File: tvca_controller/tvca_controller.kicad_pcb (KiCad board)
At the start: 2 copper layers, 84.3 x 59.2 mm, 57 parts, among them J1 Programming Header, J2 PT 1,5/ 4-5,0-H, J3 4DB-P108-02, J4 PT 1,5/ 4-5,0-H, J5 4DB-P108-02, J6 PT 1,5/ 4-5,0-H, J7 4DB-P108-02, J9 4DB-P108-02, U1 PIC18F26K83, U2 MCP2562, U3 INA180, U8 VNH7070AS, U9 VNH7070AS, Y1 Crystal 12 MHz

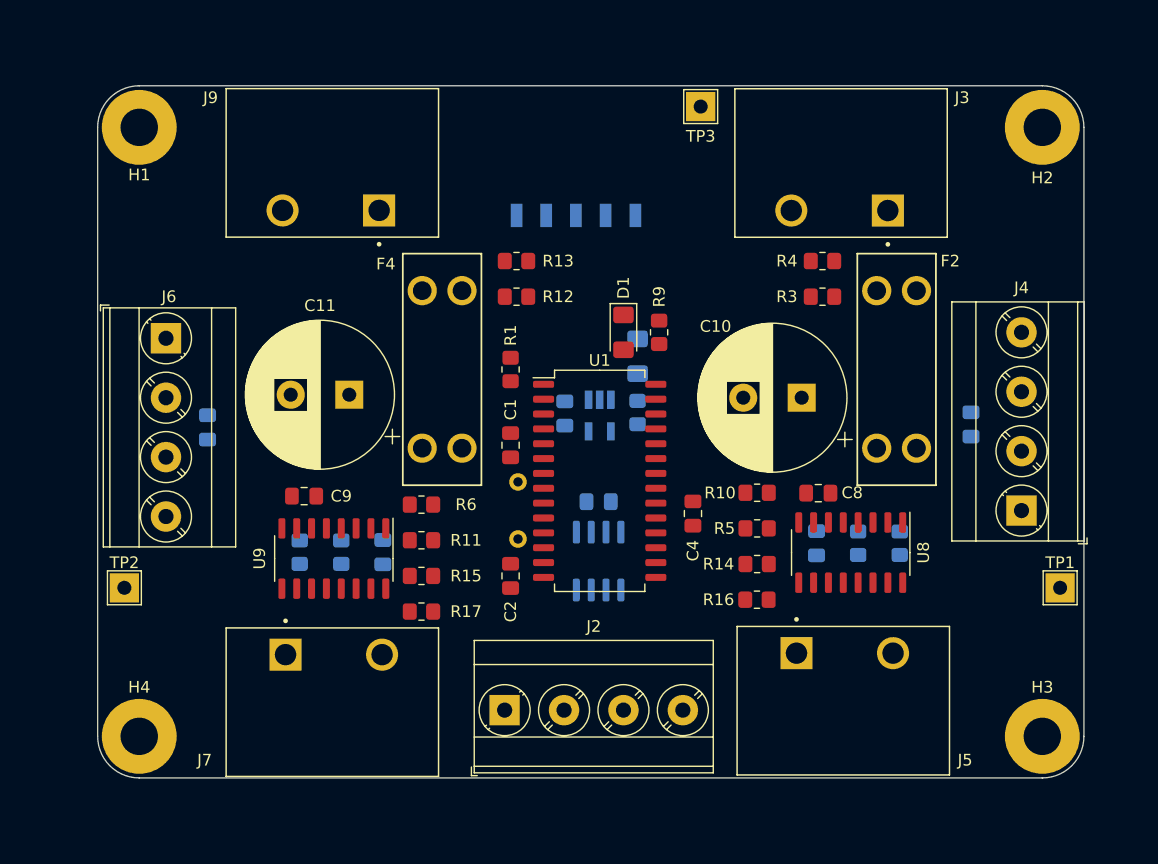
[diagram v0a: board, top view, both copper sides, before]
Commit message: High power routing
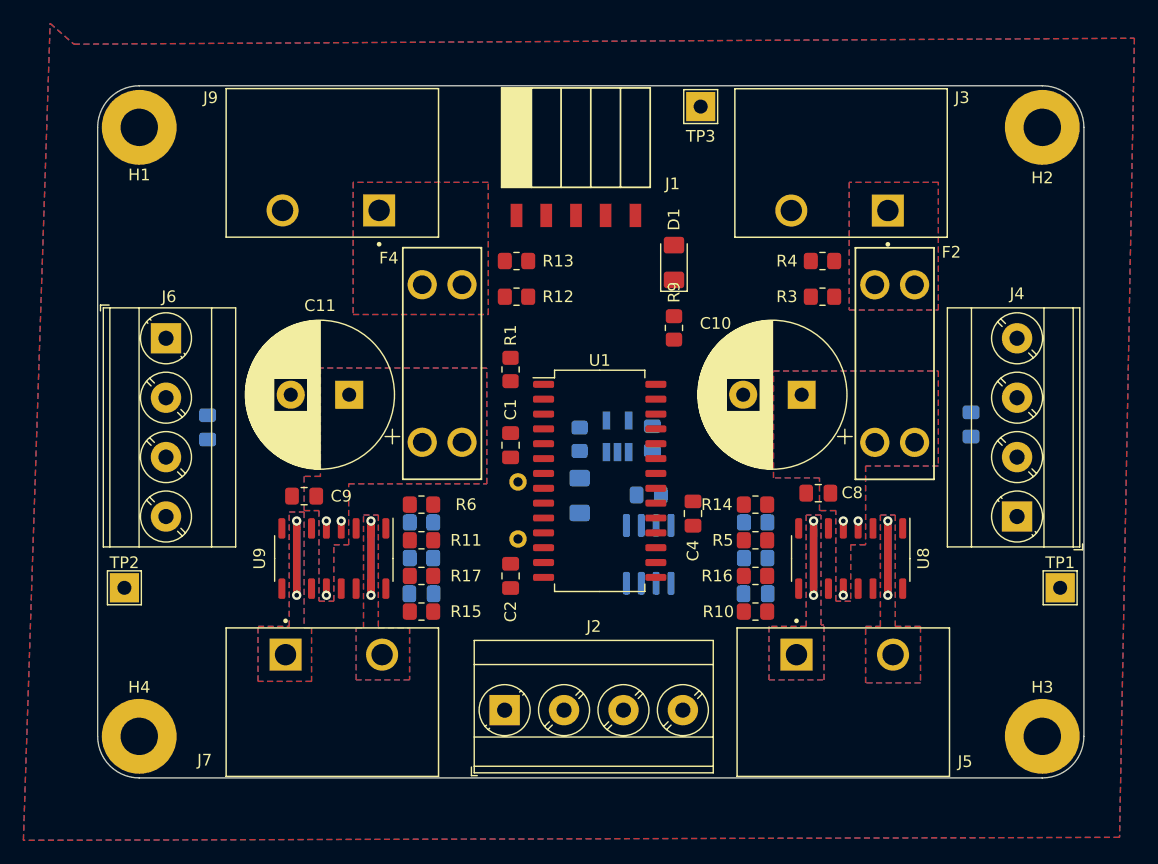
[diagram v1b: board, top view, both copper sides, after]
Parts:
- J1: moved to F.Cu
- moved F1 12.9 mm to (146.1, 110.0), turned to 90 degrees
- moved R18 12.4 mm to (161.2, 112.3), turned to 0 degrees
- moved R19 10.7 mm to (132.6, 112.3), turned to 180 degrees
- moved R10 10.2 mm to (161.1, 119.9)
- moved J1 10.2 mm to (140.7, 86.0), turned to 0 degrees
- moved R7 8.85 mm to (161.2, 115.3), turned to 180 degrees
- moved C5 7.78 mm to (152.3, 105.1), turned to -90 degrees
- moved D1 7.37 mm to (154.2, 90.0), turned to 90 degrees
- moved R8 6.88 mm to (132.6, 115.3), turned to 0 degrees
- moved C6 6.76 mm to (161.2, 118.4), turned to 0 degrees
- moved R2 5.46 mm to (146.1, 105.2), turned to -90 degrees
- moved R14 5.08 mm to (161.1, 110.7)
- moved C7 4.85 mm to (132.6, 118.4), turned to 180 degrees
- moved C3 4.32 mm to (152.0, 109.9)
- moved U2 4.32 mm to (152.0, 115.0)
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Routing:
- net /Motor_2/OUT_1: track 0.00 -> 13.6 mm, vias 0 -> 2
- net /Motor_2/OUT_2: track 0.00 -> 12.7 mm, vias 0 -> 2
- net /Motor_1/OUT_1: track 0.00 -> 12.7 mm, vias 0 -> 2
- net /Motor_1/OUT_2: track 0.00 -> 11.5 mm, vias 0 -> 2
- net /Motor_2/POWER: vias 0 -> 3
- net /Motor_1/POWER: vias 0 -> 3
- added copper zone on B.Cu, net /Motor_1/OUT_1
- added copper zone on F.Cu, net /Motor_1/OUT_1
- added copper zone on B.Cu, net /Motor_1/OUT_2
- added copper zone on F.Cu, net /Motor_1/OUT_2
- added copper zone on B.Cu, net /Motor_1/POWER
- added copper zone on F.Cu, net /Motor_1/POWER
- added copper zone on B.Cu, net /Motor_2/OUT_1
- added copper zone on F.Cu, net /Motor_2/OUT_1
- added copper zone on B.Cu, net /Motor_2/OUT_2
- added copper zone on F.Cu, net /Motor_2/OUT_2
- added copper zone on B.Cu, net /Motor_2/POWER
- added copper zone on F.Cu, net /Motor_2/POWER
- added copper zone on B.Cu, net GND
- added copper zone on F.Cu, net GND
- added copper zone on B.Cu, net Net-(J3-Pin_1)
- added copper zone on F.Cu, net Net-(J3-Pin_1)
- added copper zone on B.Cu, net Net-(J9-Pin_1)
- added copper zone on F.Cu, net Net-(J9-Pin_1)

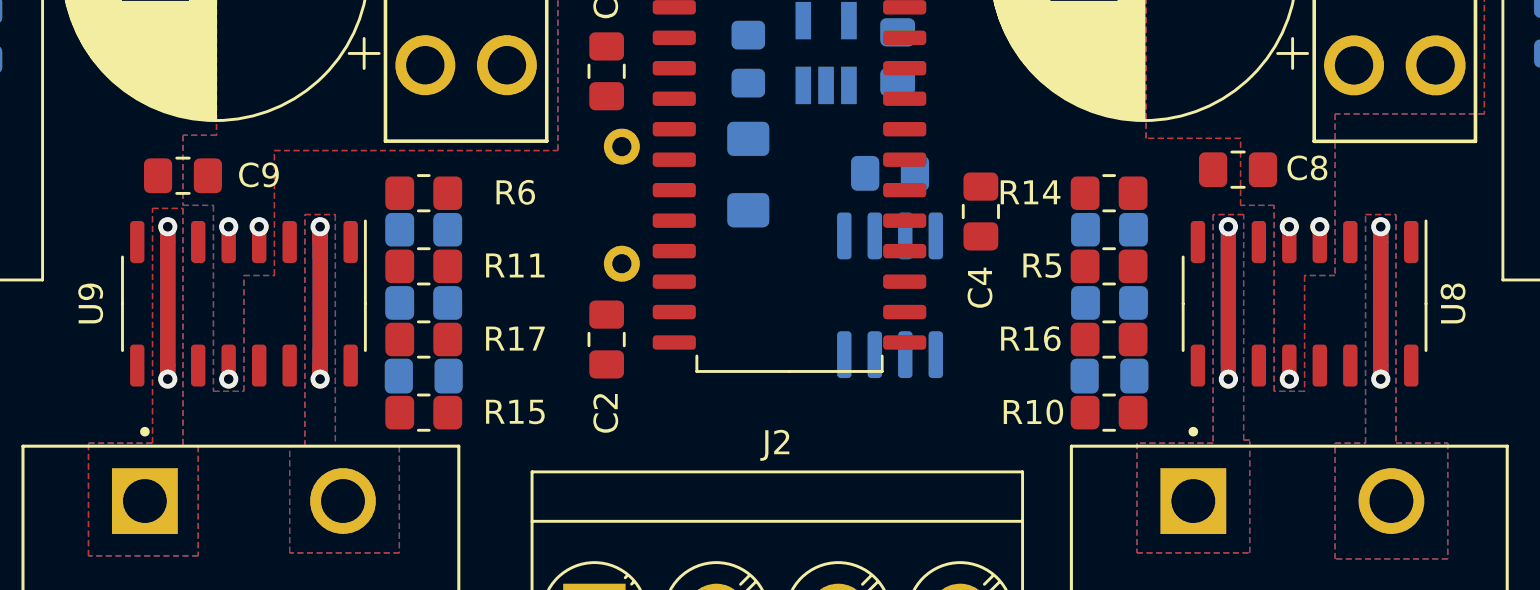
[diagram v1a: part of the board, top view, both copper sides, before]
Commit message: small fix
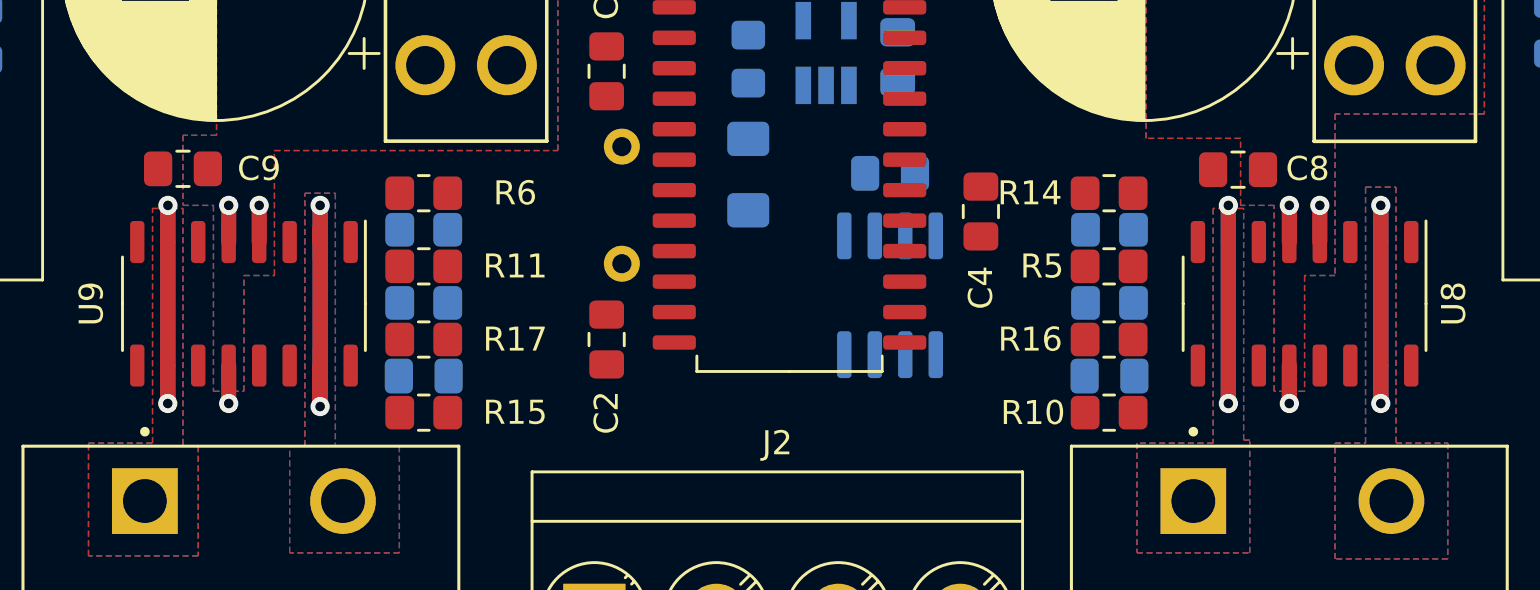
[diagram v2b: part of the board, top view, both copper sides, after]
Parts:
- moved C9 0.29 mm to (122.6, 109.7)
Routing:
- net /Motor_2/OUT_1: track 13.6 -> 19.5 mm
- net /Motor_1/OUT_2: track 11.5 -> 16.4 mm
- net /Motor_2/POWER: track 0.00 -> 4.63 mm
- net /Motor_1/POWER: track 0.00 -> 4.63 mm
- net /Motor_1/OUT_1: track 12.7 -> 16.5 mm
- net /Motor_2/OUT_2: track 12.7 -> 16.4 mm
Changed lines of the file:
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@@
   )
   (footprint "Capacitor_SMD:C_0805_2012Metric_Pad1.18x1.45mm_HandSolder" (layer "F.Cu")
-    (at 122.555 110.017 180)
+    (at 122.555 109.728 180)
     (descr "Capacitor SMD 0805 (2012 Metric), square (rectangular) end terminal, IPC_7351 nominal with elongated pad for handsoldering. (Body size source: IPC-SM-782 page 76, https://www.pcb-3d.com/wordpress/wp-content/uploads/ipc-sm-782a_amendment_1_and_2.pdf, https://docs.google.com/spreadsheets/d/1BsfQQcO9C6DZCsRaXUlFlo91Tg2WpOkGARC1WS5S8t0/edit?usp=sharing), generated with kicad-footprint-generator")
     (tags "capacitor handsolder")
@@
   (gr_arc (start 189.23 130.556) (mid 188.188472 133.070472) (end 185.674 134.112)
     (stroke (width 0.1) (type default)) (layer "Edge.Cuts"))
-  (via (at 168.656 112.141) (size 0.8) (drill 0.4) (layers "F.Cu" "B.Cu") (net 21))
-  (via (at 169.926 112.141) (size 0.8) (drill 0.4) (layers "F.Cu" "B.Cu") (net 21))
-  (via (at 168.656 118.491) (size 0.8) (drill 0.4) (layers "F.Cu" "B.Cu") (net 21))
-  (via (at 125.73 112.141) (size 0.8) (drill 0.4) (layers "F.Cu" "B.Cu") (net 22))
-  (via (at 124.46 112.141) (size 0.8) (drill 0.4) (layers "F.Cu" "B.Cu") (net 22))
-  (via (at 124.46 118.491) (size 0.8) (drill 0.4) (layers "F.Cu" "B.Cu") (net 22))
-  (segment (start 172.466 112.776) (end 172.466 112.141) (width 0.635) (layer "F.Cu") (net 43))
+  (segment (start 169.926 112.776) (end 169.926 111.252) (width 0.635) (layer "F.Cu") (net 21))
+  (segment (start 168.656 117.926) (end 168.656 119.507) (width 0.635) (layer "F.Cu") (net 21))
+  (segment (start 168.656 112.776) (end 168.656 111.252) (width 0.635) (layer "F.Cu") (net 21))
+  (via (at 168.656 111.252) (size 0.8) (drill 0.4) (layers "F.Cu" "B.Cu") (net 21))
+  (via (at 169.926 111.252) (size 0.8) (drill 0.4) (layers "F.Cu" "B.Cu") (net 21))
+  (via (at 168.656 119.507) (size 0.8) (drill 0.4) (layers "F.Cu" "B.Cu") (net 21))
+  (segment (start 124.46 117.926) (end 124.46 119.507) (width 0.635) (layer "F.Cu") (net 22))
+  (segment (start 124.46 112.776) (end 124.46 111.252) (width 0.635) (layer "F.Cu") (net 22))
+  (segment (start 125.73 112.776) (end 125.73 111.252) (width 0.635) (layer "F.Cu") (net 22))
+  (via (at 125.73 111.252) (size 0.8) (drill 0.4) (layers "F.Cu" "B.Cu") (net 22))
+  (via (at 124.46 111.252) (size 0.8) (drill 0.4) (layers "F.Cu" "B.Cu") (net 22))
+  (via (at 124.46 119.507) (size 0.8) (drill 0.4) (layers "F.Cu" "B.Cu") (net 22))
+  (segment (start 172.466 112.776) (end 172.466 111.252) (width 0.635) (layer "F.Cu") (net 43))
+  (segment (start 172.466 117.926) (end 172.466 119.507) (width 0.635) (layer "F.Cu") (net 43))
   (segment (start 172.466 112.776) (end 172.466 117.926) (width 0.635) (layer "F.Cu") (net 43))
-  (segment (start 172.466 118.491) (end 172.466 117.926) (width 0.635) (layer "F.Cu") (net 43))
-  (via (at 172.466 118.491) (size 0.8) (drill 0.4) (layers "F.Cu" "B.Cu") (net 43))
-  (via (at 172.466 112.141) (size 0.8) (drill 0.4) (layers "F.Cu" "B.Cu") (net 43))
-  (segment (start 172.466 112.141) (end 172.466 118.491) (width 0.635) (layer "B.Cu") (net 43))
+  (via (at 172.466 119.507) (size 0.8) (drill 0.4) (layers "F.Cu" "B.Cu") (net 43))
+  (via (at 172.466 111.252) (size 0.8) (drill 0.4) (layers "F.Cu" "B.Cu") (net 43))
+  (segment (start 172.466 111.252) (end 172.466 119.507) (width 0.635) (layer "B.Cu") (net 43))
   (segment (start 166.116 112.776) (end 166.116 117.926) (width 0.635) (layer "F.Cu") (net 44))
-  (via (at 166.116 112.141) (size 0.8) (drill 0.4) (layers "F.Cu" "B.Cu") (net 44))
-  (via (at 166.116 118.491) (size 0.8) (drill 0.4) (layers "F.Cu" "B.Cu") (net 44))
-  (segment (start 166.116 112.141) (end 166.116 118.491) (width 0.635) (layer "B.Cu") (net 44))
-  (segment (start 128.27 118.491) (end 128.27 117.926) (width 0.635) (layer "F.Cu") (net 45))
-  (segment (start 128.27 112.776) (end 128.27 112.268) (width 0.635) (layer "F.Cu") (net 45))
-  (segment (start 128.27 112.268) (end 128.27 118.491) (width 0.635) (layer "F.Cu") (net 45))
-  (via (at 128.27 118.491) (size 0.8) (drill 0.4) (layers "F.Cu" "B.Cu") (net 45))
-  (via (at 128.27 112.141) (size 0.8) (drill 0.4) (layers "F.Cu" "B.Cu") (net 45))
-  (segment (start 128.27 112.141) (end 128.27 118.491) (width 0.635) (layer "B.Cu") (net 45))
+  (segment (start 166.116 117.926) (end 166.116 119.507) (width 0.635) (layer "F.Cu") (net 44))
+  (segment (start 166.116 112.776) (end 166.116 111.252) (width 0.635) (layer "F.Cu") (net 44))
+  (via (at 166.116 111.252) (size 0.8) (drill 0.4) (layers "F.Cu" "B.Cu") (net 44))
+  (via (at 166.116 119.507) (size 0.8) (drill 0.4) (layers "F.Cu" "B.Cu") (net 44))
+  (segment (start 166.116 111.379) (end 166.116 119.507) (width 0.635) (layer "B.Cu") (net 44))
+  (segment (start 128.27 119.634) (end 128.27 112.268) (width 0.635) (layer "F.Cu") (net 45))
+  (segment (start 128.27 112.776) (end 128.27 111.252) (width 0.635) (layer "F.Cu") (net 45))
+  (segment (start 128.27 112.268) (end 128.27 112.776) (width 0.635) (layer "F.Cu") (net 45))
+  (segment (start 128.27 117.926) (end 128.27 119.634) (width 0.635) (layer "F.Cu") (net 45))
+  (via (at 128.27 119.634) (size 0.8) (drill 0.4) (layers "F.Cu" "B.Cu") (net 45))
+  (via (at 128.27 111.252) (size 0.8) (drill 0.4) (layers "F.Cu" "B.Cu") (net 45))
+  (segment (start 128.27 111.252) (end 128.27 119.634) (width 0.635) (layer "B.Cu") (net 45))
   (segment (start 121.92 112.776) (end 121.92 117.926) (width 0.635) (layer "F.Cu") (net 46))
-  (segment (start 121.92 112.776) (end 121.92 112.141) (width 0.635) (layer "F.Cu") (net 46))
-  (segment (start 121.92 118.491) (end 121.92 117.926) (width 0.635) (layer "F.Cu") (net 46))
-  (via (at 121.92 112.141) (size 0.8) (drill 0.4) (layers "F.Cu" "B.Cu") (net 46))
-  (via (at 121.92 118.491) (size 0.8) (drill 0.4) (layers "F.Cu" "B.Cu") (net 46))
-  (segment (start 121.92 112.141) (end 121.92 118.491) (width 0.635) (layer "B.Cu") (net 46))
+  (segment (start 121.92739 111.338411) (end 121.92 111.345801) (width 0.635) (layer "F.Cu") (net 46))
+  (segment (start 121.92 112.776) (end 121.92 111.25939) (width 0.635) (layer "F.Cu") (net 46))
+  (segment (start 121.92 111.25939) (end 121.92739 111.252) (width 0.635) (layer "F.Cu") (net 46))
+  (segment (start 121.92 117.926) (end 121.92 119.507) (width 0.635) (layer "F.Cu") (net 46))
+  (via (at 121.92739 111.252) (size 0.8) (drill 0.4) (layers "F.Cu" "B.Cu") (net 46))
+  (via (at 121.92 119.507) (size 0.8) (drill 0.4) (layers "F.Cu" "B.Cu") (net 46))
+  (segment (start 121.92739 111.338411) (end 121.92 111.345801) (width 0.635) (layer "B.Cu") (net 46))
+  (segment (start 121.92 111.345801) (end 121.92 119.507) (width 0.635) (layer "B.Cu") (net 46))
   (zone (net 43) (net_name "/Motor_1/OUT_1") (layers "F&B.Cu") (hatch edge 0.5)
     (priority 8)
@@
     (polygon
       (pts
-        (xy 171.831 111.633)
-        (xy 173.101 111.633)
+        (xy 171.831 110.49)
+        (xy 173.101 110.49)
         (xy 173.101 121.158)
         (xy 175.26 121.158)
@@
     (polygon
       (pts
-        (xy 165.481 111.633)
+        (xy 165.481 111.379)
         (xy 165.481 121.158)
         (xy 162.306 121.158)
@@
         (xy 167.005 121.031)
         (xy 166.751 121.031)
-        (xy 166.751 111.633)
+        (xy 166.751 111.379)
       )
     )
@@
     (polygon
       (pts
-        (xy 127.635 111.633)
-        (xy 128.905 111.633)
+        (xy 127.635 110.744)
+        (xy 128.905 110.744)
         (xy 128.905 121.285)
         (xy 131.572 121.285)
